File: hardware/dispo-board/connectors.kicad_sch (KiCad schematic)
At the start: 19 parts, among them J1 USB_B_Micro, J10 Conn_01x02, J11 Conn_01x02, J2 Conn_01x03, J3 Conn_01x03, J4 Conn_01x03, J5 Conn_01x02, J6 Conn_01x02, J7 Conn_01x02, J8 Conn_01x02, J9 Conn_01x04

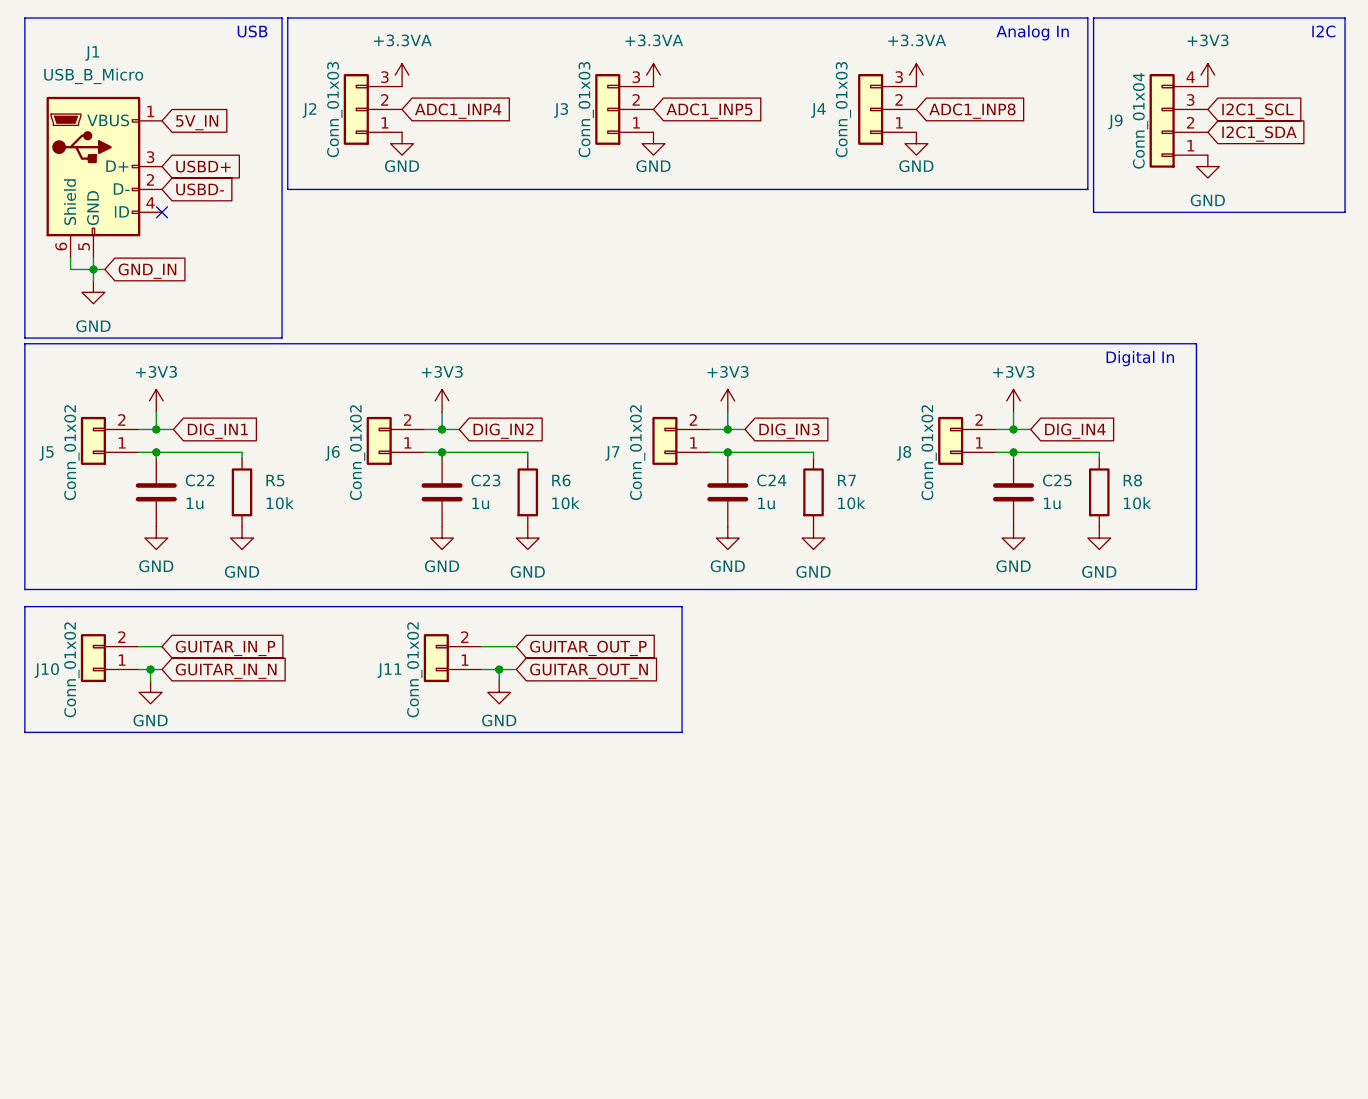
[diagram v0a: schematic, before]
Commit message: maybe final schematic?
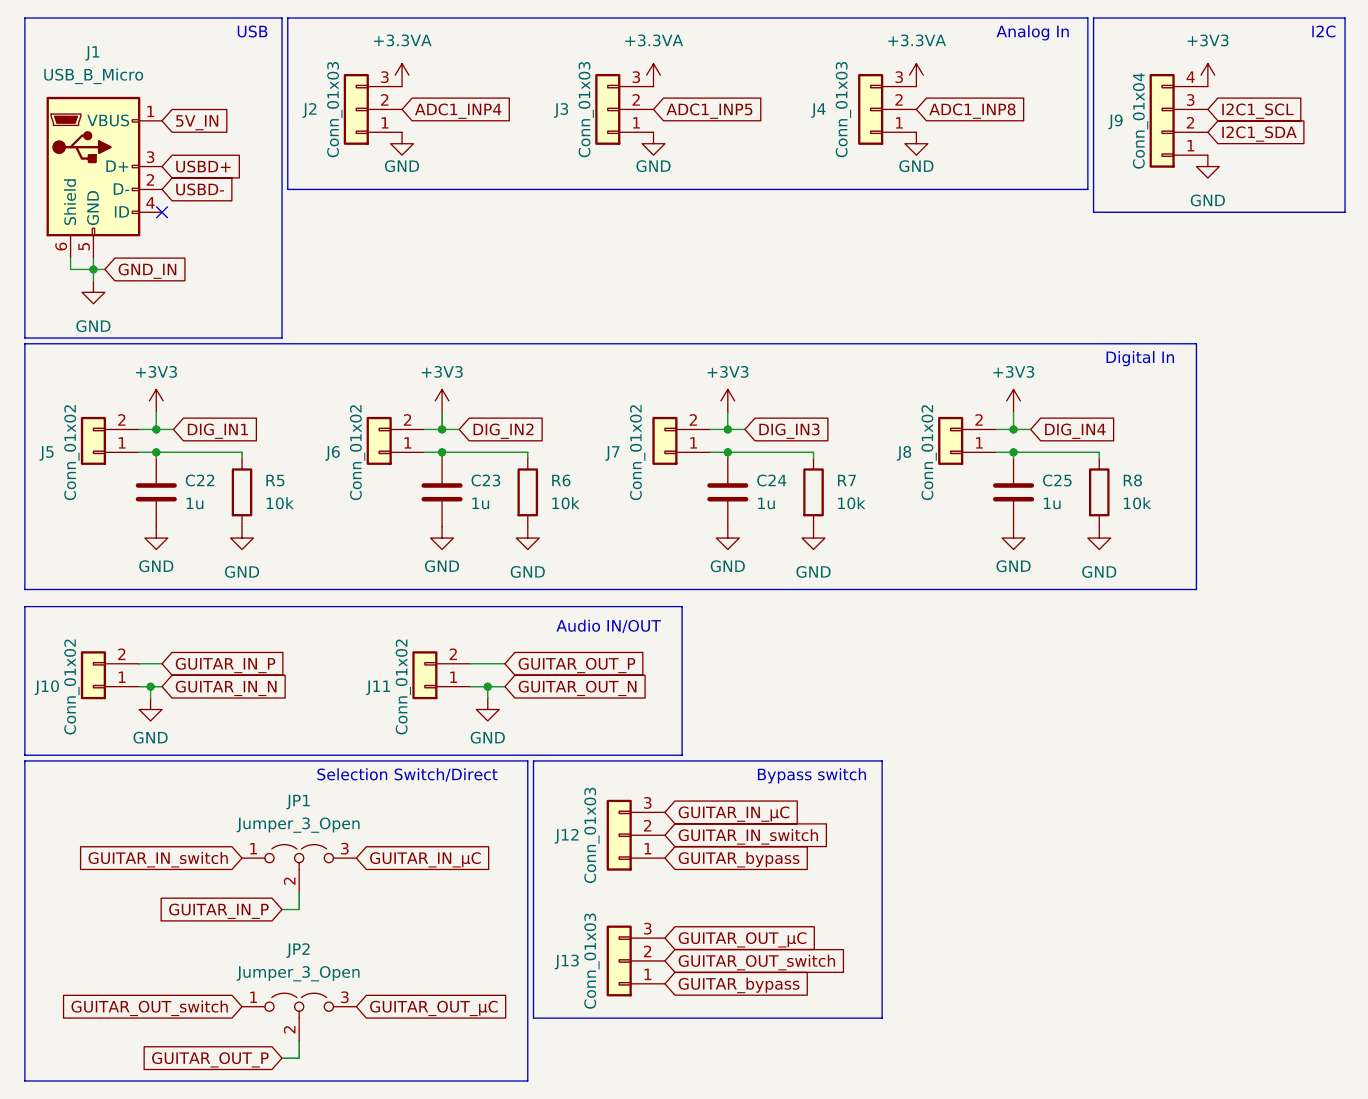
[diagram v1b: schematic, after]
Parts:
- added J12, J13: Conn_01x03, MyFootprints:solder_pad_1x3_D2.00mm, symbol Connector_Generic:Conn_01x03
- added JP1, JP2: Jumper_3_Open, symbol Jumper:Jumper_3_Open
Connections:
- net GUITAR_IN_P: now also JP1.2 (C)
- net GUITAR_OUT_P: now also JP2.2 (C)
- new net GUITAR_IN_switch: J12.2 (Pin_2), JP1.1 (A)
- new net GUITAR_IN_µC: J12.3 (Pin_3), JP1.3 (B)
- new net GUITAR_OUT_switch: J13.2 (Pin_2), JP2.1 (A)
- new net GUITAR_OUT_µC: J13.3 (Pin_3), JP2.3 (B)
- new net GUITAR_bypass: J12.1 (Pin_1), J13.1 (Pin_1)
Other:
- note added: "Audio IN/OUT"
- note added: "Bypass switch"
- note added: "Selection Switch/Direct"
- moved on the sheet: J10, J11
